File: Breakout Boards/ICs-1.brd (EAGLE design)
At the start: 75 x 70 mm, 26 parts

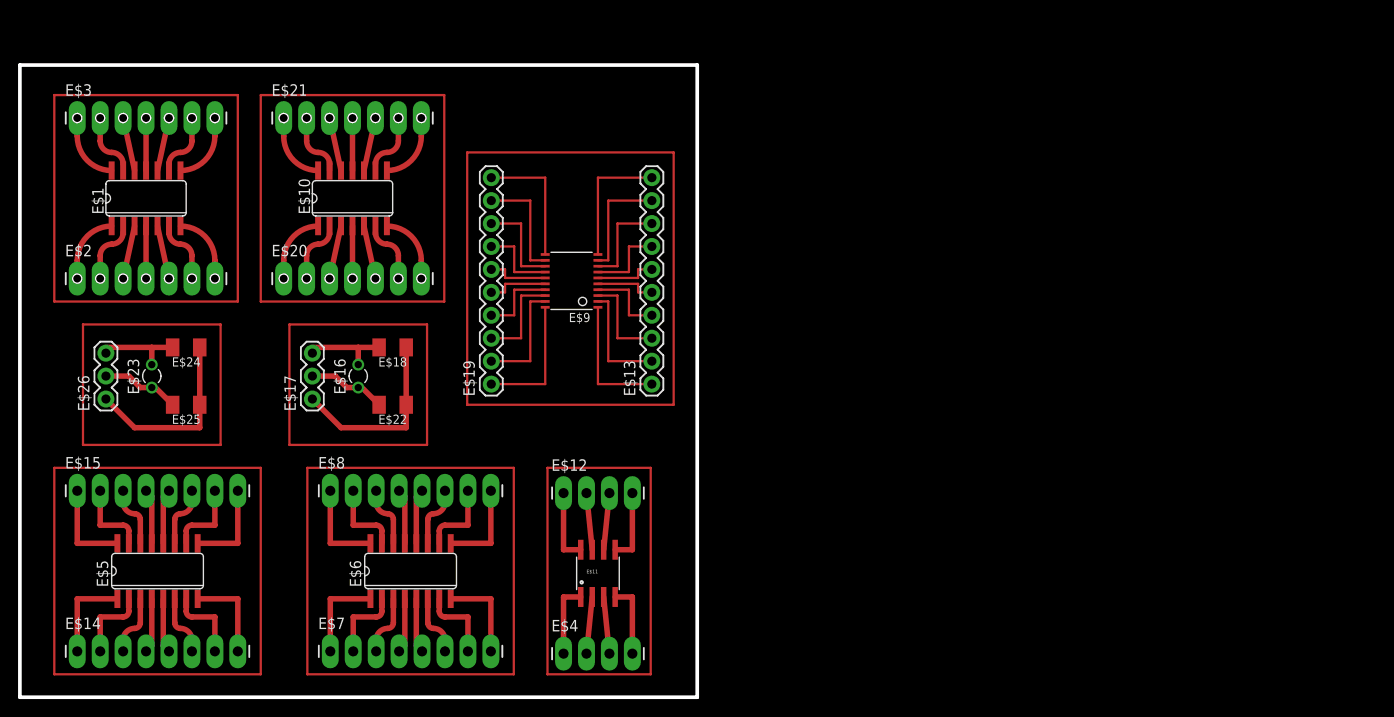
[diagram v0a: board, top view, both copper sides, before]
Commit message: breakout board update
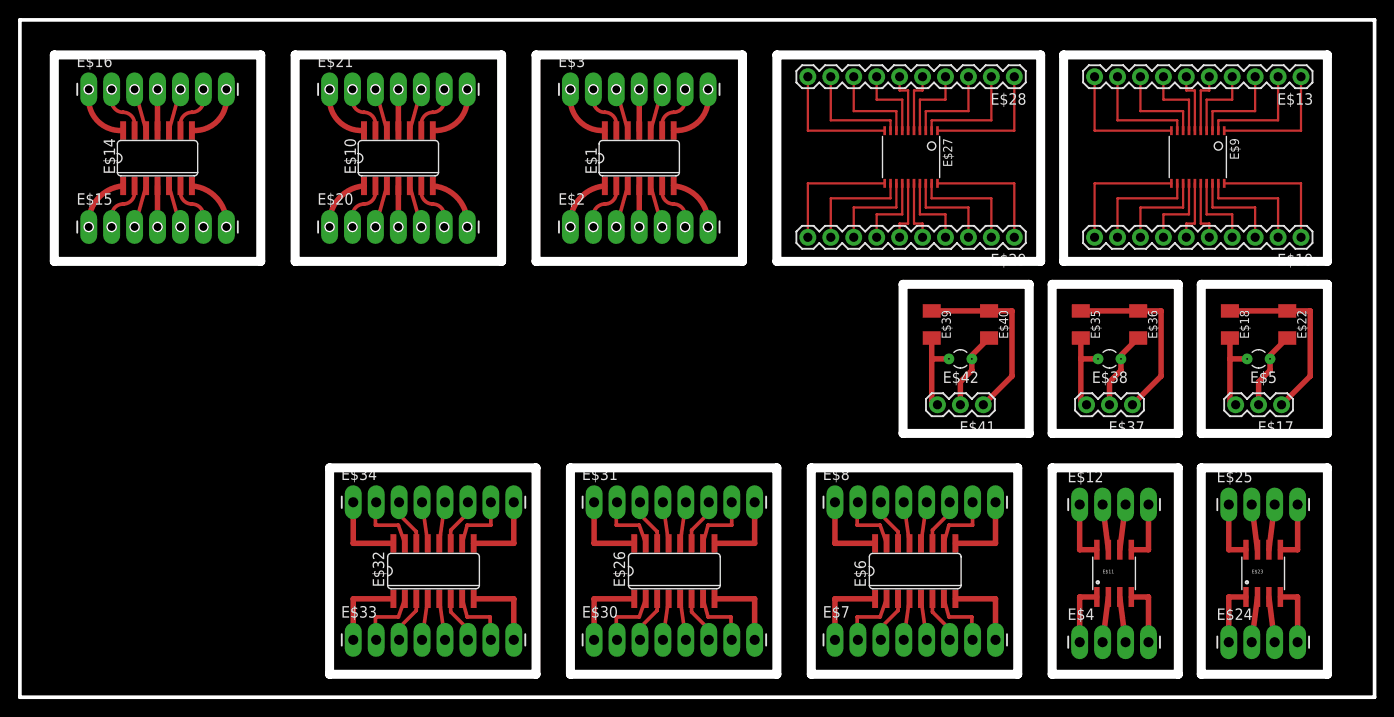
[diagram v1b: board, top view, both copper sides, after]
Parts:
- added E$27: (no value), iStivi - ICs:TSSOP20
- added E$28, E$29: (no value), iStivi - Header-Connector:1X10
- added E$30, E$31, E$33, E$34: (no value), iStivi - Header-Connector:1X08_LONGPADS
- added E$32: (no value), iStivi - ICs:SO16
- added E$35, E$36, E$39, E$40: (no value), iStivi - RCLD:C1206K
- added E$37, E$41: (no value), iStivi - Header-Connector:1X03
- added E$38, E$42: (no value), iStivi - Oscillators:TC26V
- E$14: device iStivi - Header-Connector:1X08_LONGPADS -> iStivi - ICs:SO14
- E$15: device iStivi - Header-Connector:1X08_LONGPADS -> iStivi - Header-Connector:1X07_LONGPADS
- E$16: device iStivi - Oscillators:TC26V -> iStivi - Header-Connector:1X07_LONGPADS
- E$23: device iStivi - Oscillators:TC26V -> iStivi - ICs:SO08
- E$24, E$25: device iStivi - RCLD:C1206K -> iStivi - Header-Connector:1X04_LONGPADS
- E$26: device iStivi - Header-Connector:1X03 -> iStivi - ICs:SO16
- E$5: device iStivi - ICs:SO16 -> iStivi - Oscillators:TC26V
- moved E$23 125.0 mm to (137.7, 13.7), turned to 0 degrees
- moved E$5 124.2 mm to (137.2, 37.5), turned to 180 degrees
- moved E$24 120.0 mm to (133.9, 6.10), turned to 0 degrees
- moved E$25 116.0 mm to (133.9, 21.3), turned to 0 degrees
- moved E$17 107.3 mm to (139.7, 32.4), turned to 180 degrees
- moved E$22 99.5 mm to (140.3, 41.3), turned to 270 degrees
- moved E$18 92.7 mm to (134.0, 41.3), turned to 270 degrees
- moved E$19 91.1 mm to (141.9, 50.9), turned to 180 degrees
- moved E$13 79.5 mm to (141.9, 68.7), turned to 180 degrees
- moved E$9 70.7 mm to (130.4, 59.8), turned to 180 degrees
- moved E$26 65.8 mm to (72.5, 14.0), turned to 0 degrees
- moved E$12 57.2 mm to (117.3, 21.3)
- moved E$4 57.2 mm to (117.3, 6.10)
- moved E$11 57.2 mm to (121.2, 13.7)
- moved E$7 55.9 mm to (90.2, 6.35)
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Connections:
- removed net S$38: E$23.1, E$25.2, E$26.2
- new net S$105: E$23.3, E$24.3
- new net S$106: E$23.4, E$24.4
- new net S$107: E$27.9, E$28.9
- new net S$108: E$26.16, E$31.1
- new net S$109: E$26.15, E$31.2
- new net S$110: E$26.14, E$31.3
- new net S$111: E$26.13, E$31.4
- new net S$112: E$27.10, E$28.10
- new net S$113: E$27.20, E$29.1
- new net S$114: E$27.19, E$29.2
- new net S$115: E$27.18, E$29.3
- new net S$116: E$27.17, E$29.4
- new net S$117: E$27.16, E$29.5
- new net S$118: E$27.15, E$29.6
- new net S$119: E$27.14, E$29.7
- new net S$120: E$27.12, E$29.9
- new net S$121: E$27.13, E$29.8
- new net S$122: E$27.11, E$29.10
- new net S$123: E$26.12, E$31.5
- new net S$124: E$26.11, E$31.6
- new net S$125: E$26.10, E$31.7
- new net S$126: E$26.9, E$31.8
- new net S$127: E$26.1, E$30.1
- new net S$128: E$26.2, E$30.2
- new net S$129: E$26.3, E$30.3
- new net S$130: E$26.4, E$30.4
- new net S$131: E$26.5, E$30.5
- new net S$132: E$26.7, E$30.7
- new net S$133: E$26.6, E$30.6
- new net S$134: E$26.8, E$30.8
- new net S$135: E$32.16, E$34.1
- new net S$136: E$32.15, E$34.2
- new net S$137: E$32.14, E$34.3
- new net S$138: E$32.13, E$34.4
- new net S$139: E$32.12, E$34.5
- new net S$140: E$32.11, E$34.6
- new net S$141: E$32.10, E$34.7
- new net S$142: E$32.9, E$34.8
- new net S$143: E$32.1, E$33.1
- new net S$144: E$32.2, E$33.2
- new net S$145: E$32.3, E$33.3
- new net S$146: E$32.4, E$33.4
- new net S$147: E$32.5, E$33.5
- new net S$148: E$32.7, E$33.7
- new net S$149: E$32.6, E$33.6
- new net S$150: E$32.8, E$33.8
- new net S$151: E$35.2, E$37.3
- new net S$152: E$36.2, E$37.2
- new net S$153: E$35.1, E$36.1, E$37.1
- new net S$154: E$39.2, E$41.3
- new net S$155: E$40.2, E$41.2
- new net S$156: E$39.1, E$40.1, E$41.1
- new net S$36: E$14.3, E$15.3
- new net S$40: E$14.6, E$15.6
- new net S$41: E$27.1, E$28.1
- new net S$42: E$27.2, E$28.2
- new net S$43: E$27.3, E$28.3
- new net S$44: E$27.4, E$28.4
- new net S$45: E$27.5, E$28.5
- new net S$46: E$27.6, E$28.6
- new net S$47: E$27.7, E$28.7
- new net S$48: E$27.8, E$28.8
- net S$1: now also E$1.1, E$2.1; no longer E$15.1, E$5.16
- net S$10: now also E$1.12, E$3.3; no longer E$14.2, E$5.2
- net S$11: now also E$1.11, E$3.4; no longer E$14.3, E$5.3
- net S$12: now also E$1.10, E$3.5; no longer E$14.4, E$5.4
- net S$13: now also E$1.9, E$3.6; no longer E$14.5, E$5.5
- net S$14: now also E$1.8, E$3.7; no longer E$14.7, E$5.7
- net S$15: now also E$14.1, E$15.1; no longer E$14.6, E$5.6
- net S$16: now also E$14.2, E$15.2; no longer E$14.8, E$5.8
- net S$2: now also E$1.2, E$2.2; no longer E$15.2, E$5.15
- net S$3: now also E$1.3, E$2.3; no longer E$15.3, E$5.14
- net S$33: no longer E$16.2
- net S$34: no longer E$16.1
- net S$37: now also E$14.4, E$15.4; no longer E$23.2, E$24.2, E$26.3
- net S$39: now also E$14.5, E$15.5; no longer E$24.1, E$25.1, E$26.1
- net S$4: now also E$1.4, E$2.4; no longer E$15.4, E$5.13
- net S$49: now also E$14.7, E$15.7; no longer E$1.1, E$2.1
- net S$5: now also E$1.5, E$2.5; no longer E$15.5, E$5.12
- net S$50: now also E$14.14, E$16.1; no longer E$1.2, E$2.2
- net S$51: now also E$14.13, E$16.2; no longer E$1.3, E$2.3
- net S$52: now also E$14.12, E$16.3; no longer E$1.4, E$2.4
- net S$53: now also E$14.11, E$16.4; no longer E$1.5, E$2.5
- net S$54: now also E$14.10, E$16.5; no longer E$1.6, E$2.6
- net S$55: now also E$14.9, E$16.6; no longer E$1.7, E$2.7
- net S$56: now also E$14.8, E$16.7; no longer E$1.14, E$3.1
- net S$57: now also E$23.8, E$25.1; no longer E$1.13, E$3.2
- net S$58: now also E$23.7, E$25.2; no longer E$1.12, E$3.3
- net S$59: now also E$23.6, E$25.3; no longer E$1.11, E$3.4
- net S$6: now also E$1.6, E$2.6; no longer E$15.6, E$5.11
- net S$60: now also E$23.5, E$25.4; no longer E$1.10, E$3.5
- net S$61: now also E$23.1, E$24.1; no longer E$1.9, E$3.6
- net S$62: now also E$23.2, E$24.2; no longer E$1.8, E$3.7
- net S$7: now also E$1.7, E$2.7; no longer E$15.7, E$5.10
- net S$8: now also E$1.14, E$3.1; no longer E$15.8, E$5.9
- net S$9: now also E$1.13, E$3.2; no longer E$14.1, E$5.1
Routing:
- net S$111: track 101.6 -> 4.59 mm
- net S$105: track 91.4 -> 5.04 mm
- net S$106: track 91.4 -> 6.91 mm
- net S$109: track 86.4 -> 7.21 mm
- net S$108: track 86.4 -> 8.99 mm
- net S$110: track 68.6 -> 5.40 mm
- net S$36: track 57.1 -> 4.72 mm
- net S$40: track 57.1 -> 5.60 mm
- net S$156: track 0.00 -> 20.6 mm
- net S$153: track 0.00 -> 20.6 mm
- net S$39: track 20.6 -> 4.72 mm
- net S$122: track 0.00 -> 14.5 mm
- net S$112: track 0.00 -> 14.5 mm
- net S$113: track 0.00 -> 14.5 mm
- net S$41: track 0.00 -> 14.5 mm
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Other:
- board size 75 x 70 mm -> 150 x 75 mm

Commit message: finished
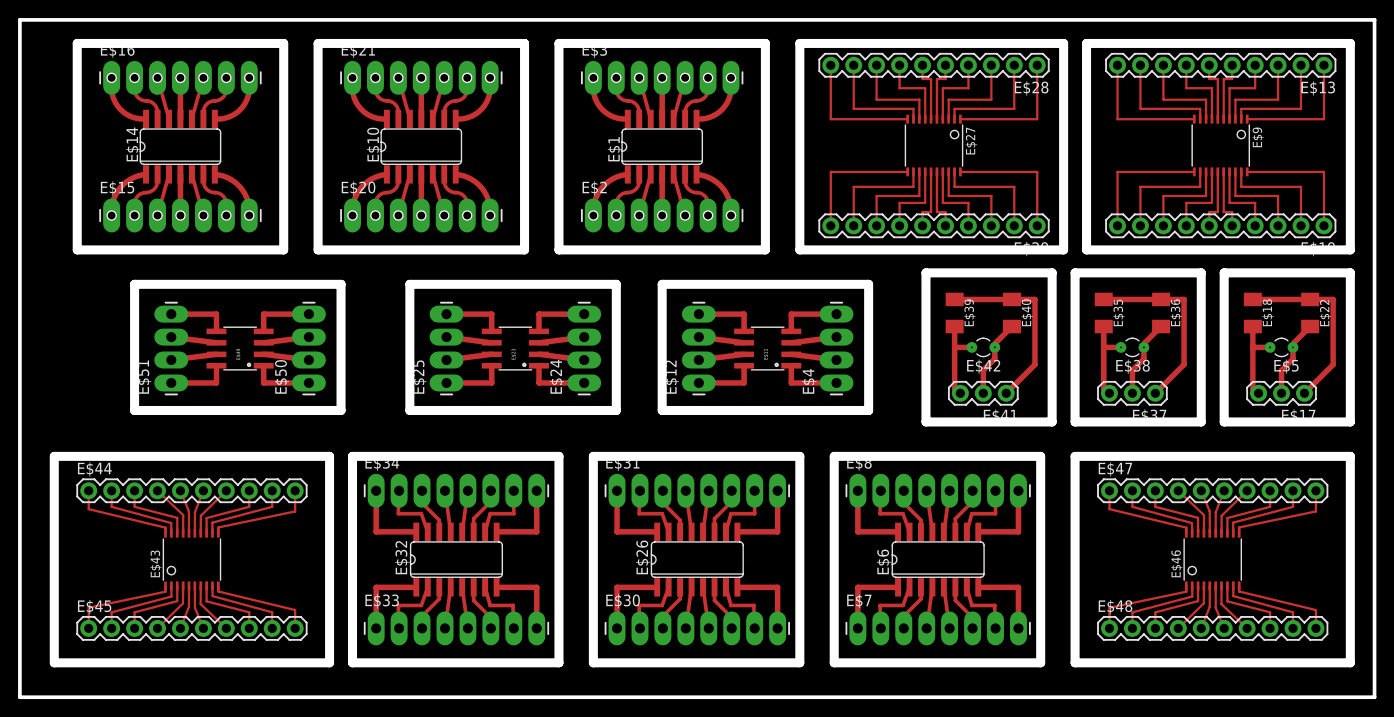
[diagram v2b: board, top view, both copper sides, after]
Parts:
- added E$43, E$46: (no value), iStivi - ICs:TSSOP20
- added E$44, E$45, E$47, E$48: (no value), iStivi - Header-Connector:1X10
- added E$49: (no value), iStivi - ICs:SO08
- added E$50, E$51: (no value), iStivi - Header-Connector:1X04_LONGPADS
- moved E$25 87.7 mm to (47.2, 34.8), turned to 90 degrees
- moved E$23 86.5 mm to (54.9, 38.6), turned to 90 degrees
- moved E$24 76.9 mm to (62.5, 34.8), turned to 90 degrees
- moved E$11 45.7 mm to (82.8, 38.6), turned to 90 degrees
- moved E$12 44.3 mm to (75.2, 34.8), turned to 90 degrees
- moved E$4 39.4 mm to (90.4, 34.8), turned to 90 degrees
- moved E$17 2.84 mm to (142.2, 33.7)
- moved E$28 2.84 mm to (112.6, 70.0)
- moved E$1 2.84 mm to (71.1, 61.0)
- moved E$10 2.84 mm to (44.5, 61.0)
- moved E$29 2.84 mm to (112.6, 52.2)
- moved E$35 2.84 mm to (120.0, 42.5)
- moved E$37 2.84 mm to (125.7, 33.7)
- moved E$40 2.84 mm to (109.9, 42.5)
- moved E$30 2.84 mm to (66.1, 7.62)
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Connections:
- new net S$157: E$43.20, E$44.1
- new net S$158: E$43.19, E$44.2
- new net S$159: E$43.18, E$44.3
- new net S$160: E$43.17, E$44.4
- new net S$161: E$43.16, E$44.5
- new net S$162: E$43.15, E$44.6
- new net S$163: E$43.14, E$44.7
- new net S$164: E$43.12, E$44.9
- new net S$165: E$43.13, E$44.8
- new net S$166: E$43.11, E$44.10
- new net S$167: E$46.20, E$47.1
- new net S$168: E$46.19, E$47.2
- new net S$169: E$46.18, E$47.3
- new net S$170: E$46.17, E$47.4
- new net S$171: E$46.16, E$47.5
- new net S$172: E$46.15, E$47.6
- new net S$173: E$46.14, E$47.7
- new net S$174: E$46.12, E$47.9
- new net S$175: E$46.13, E$47.8
- new net S$176: E$46.11, E$47.10
- new net S$197: E$49.8, E$51.1
- new net S$198: E$49.7, E$51.2
- new net S$199: E$49.6, E$51.3
- new net S$200: E$49.5, E$51.4
- new net S$201: E$49.1, E$50.1
- new net S$202: E$49.2, E$50.2
- new net S$203: E$49.3, E$50.3
- new net S$204: E$49.4, E$50.4
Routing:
- net S$186: track 0.00 -> 11.6 mm
- net S$166: track 0.00 -> 11.6 mm
- net S$196: track 0.00 -> 11.6 mm
- net S$176: track 0.00 -> 11.6 mm
- net S$177: track 0.00 -> 11.4 mm
- net S$157: track 0.00 -> 11.4 mm
- net S$187: track 0.00 -> 11.4 mm
- net S$167: track 0.00 -> 11.4 mm
- net S$194: track 0.00 -> 9.81 mm
- net S$184: track 0.00 -> 9.81 mm
- net S$174: track 0.00 -> 9.81 mm
- net S$164: track 0.00 -> 9.81 mm
- net S$168: track 0.00 -> 9.74 mm
- net S$178: track 0.00 -> 9.74 mm
- net S$158: track 0.00 -> 9.74 mm
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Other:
- outline, holes or cut-outs redrawn
